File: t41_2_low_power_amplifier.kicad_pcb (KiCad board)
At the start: 2 copper layers, 75.8 x 76.2 mm, 62 parts, among them J1 5-1814832-1, J2 5-1814832-1, J3 B2B-XH-A_LF__SN_, J5 Screw_Terminal_01x02, Q1 Q_NPN_BCE, Q10 Q_NPN_BEC, Q2 Q_NPN_BEC, Q3 Q_PMOS_GSD, Q4 Q_NPN_BCE, Q5 Q_PMOS_GSD, Q6 Q_NPN_BEC, Q7 Q_NPN_BEC, Q8 Q_NPN_BEC, Q9 Q_NPN_BEC, T1 Transformer_1P_SS, T3 Transformer_1P_SS, U1 MCP1802x-xx02xOT

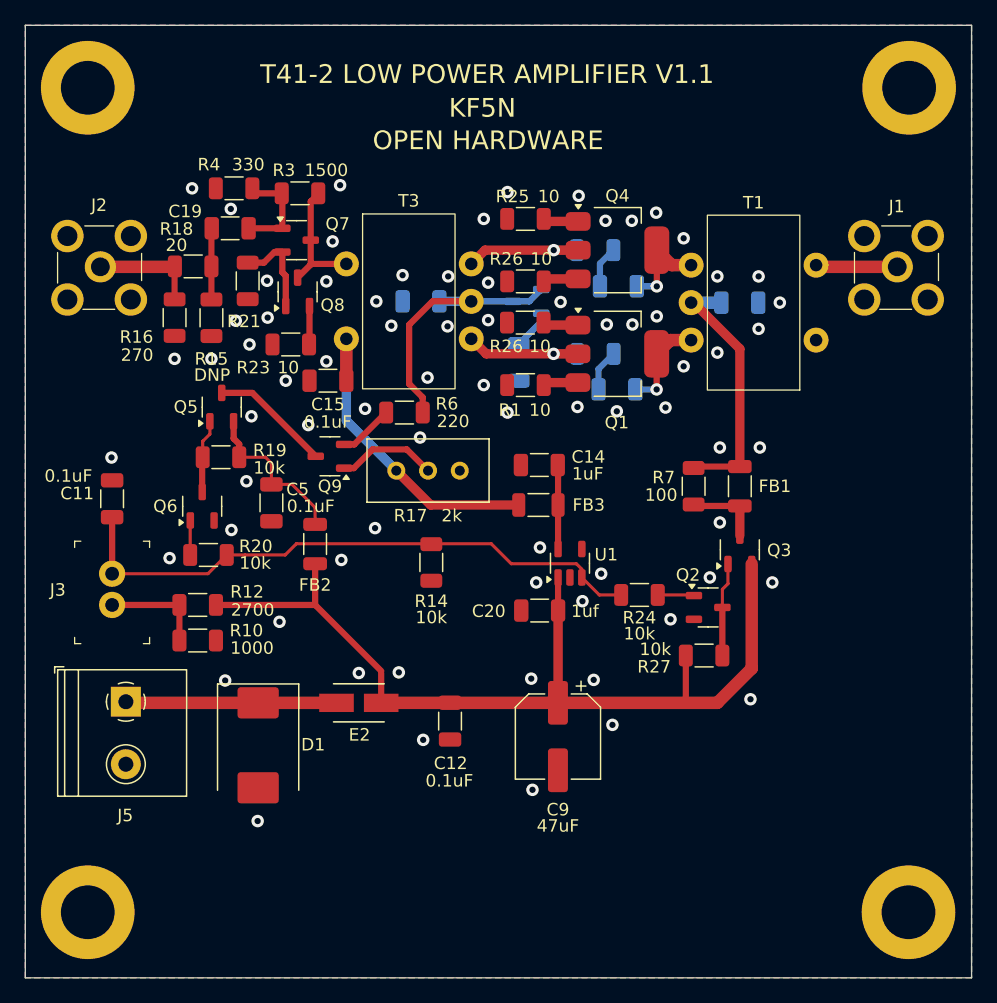
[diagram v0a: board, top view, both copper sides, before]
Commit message: T41-2 Low Power Amplifier to fab.
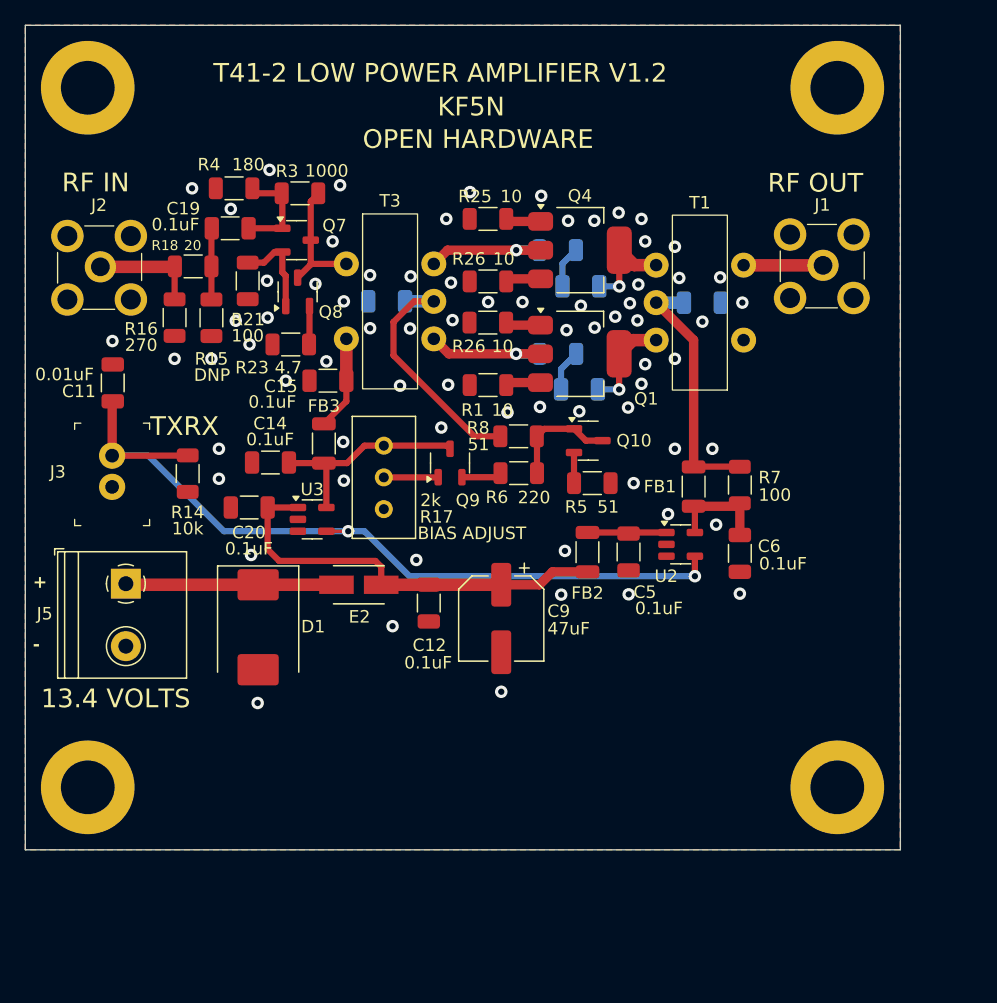
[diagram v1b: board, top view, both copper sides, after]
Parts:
- removed Q2, Q6: Q_NPN_BEC, Package_TO_SOT_SMD:SOT-23-3
- removed Q3, Q5: Q_PMOS_GSD, Package_TO_SOT_SMD:SOT-23-3
- removed R10: 1000, Resistor_SMD:R_1206_3216Metric
- removed R12: 2700, Resistor_SMD:R_1206_3216Metric
- removed R19, R20, R24, R27: 10k, Resistor_SMD:R_1206_3216Metric
- removed U1: MCP1802x-xx02xOT, Package_TO_SOT_SMD:SOT-23-5
- added C6: 0.1uF, Capacitor_SMD:C_1206_3216Metric, F.Cu at (157.2, 92.3)
- added R8: 51, Resistor_SMD:R_1206_3216Metric, F.Cu at (139.5, 82.9)
- added U2: MCP1804x-C002xOT, Package_TO_SOT_SMD:SOT-23-5, F.Cu at (152.5, 91.5)
- added U3: MCP1804x-A002xOT, Package_TO_SOT_SMD:SOT-23-5, F.Cu at (123.0, 89.5)
- C11: value 0.1uF -> 0.01uF
- C14: value 1uF -> 0.1uF
- C20: value 1uf -> 0.1uF
- Q10, R5: moved to F.Cu
- R23: value 10 -> 4.7
- R3: value 1500 -> 1000
- R4: value 330 -> 180
- moved C5 28.9 mm to (148.3, 92.2)
- moved C20 24.7 mm to (117.9, 88.6)
- moved FB2 21.8 mm to (145.0, 92.2)
- moved C14 21.5 mm to (119.6, 85.0)
- moved R14 20.8 mm to (113.0, 85.9)
- moved FB3 17.9 mm to (123.9, 83.5), turned to 90 degrees
- moved Q10 12.2 mm to (145.1, 83.2), turned to 0 degrees
- moved H3 11.5 mm to (165.0, 111.0)
- moved R5 11.3 mm to (145.4, 86.7), turned to 180 degrees
- moved C9 10.5 mm to (138.1, 97.5)
- moved R6 10.4 mm to (139.5, 85.8)
- moved H2 10.0 mm to (105.0, 111.0)
- moved Q9 9.63 mm to (134.0, 85.0), turned to 90 degrees
- moved C12 9.60 mm to (132.3, 96.2)
- moved D1 9.45 mm to (118.6, 98.2)
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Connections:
- net Net-(Q3-D) renamed /12V_REG
- C14 pad 1: Net-(U1-VOUT) -> /10V_FIL
- FB3 pad 1: Net-(U1-VOUT) -> /10V_FIL
- J3 pad 2: Net-(J3-Pad2) -> GND
- Q10 pad 1: /BASE_BIAS -> Net-(Q10-B)
- Q10 pad 3: /BASE_BIAS -> Net-(Q10-B)
- Q9 pad 3: /12V_IN_FIL -> /10V_FIL
- R17 pad 1: /10V_REG -> /10V_FIL
- R6 pad 1: /BASE_BIAS -> Net-(Q10-B)
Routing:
- net /12V: track 74.3 -> 33.8 mm
- net /10V_REG: track 26.5 -> 7.55 mm
- net /10V_FIL: track 0.00 -> 17.2 mm
- net /TXRX: track 48.5 -> 64.4 mm, vias 0 -> 2
- net /12V_IN_FIL: track 9.68 -> 0.00 mm
- net Net-(Q10-B): track 0.00 -> 8.85 mm
- net Net-(J3-Pad2): track 8.24 -> 0.00 mm
- net Net-(Q2-C): track 7.51 -> 0.00 mm
- net Net-(U2-VIN): track 13.2 -> 6.27 mm
- net Net-(U1-VOUT): track 6.04 -> 0.00 mm
- net Net-(Q5-G): track 5.97 -> 0.00 mm
- net Net-(Q9-B): track 8.04 -> 4.36 mm
- net Net-(Q2-B): track 2.92 -> 0.00 mm
- net Net-(Q6-B): track 2.77 -> 0.00 mm
- net /12V_REG: track 6.12 -> 8.77 mm
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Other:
- board size 75.8 x 76.2 mm -> 70.1 x 66 mm
- board text added: "+"
- board text added: "-"
- board text added: "13.4 VOLTS"
- board text added: "BIAS ADJUST"
- board text added: "RF IN"
- board text added: "RF OUT"
- board text added: "T41-2 LOW POWER AMPLIFIER V1.2"
- board text added: "TXRX"
- board text removed: "T41-2 LOW POWER AMPLIFIER V1.1"
